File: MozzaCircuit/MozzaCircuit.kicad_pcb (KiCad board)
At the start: 2 copper layers, 183 x 128.1 mm, 174 parts, among them J1 8P8C_both_sides, SW13 SW_ChocV2_rev, SW14 SW_ChocV2_rev, SW15 SW_ChocV2_rev, SW21 SW_ChocV2_rev, SW22 SW_ChocV2_rev, SW23 SW_ChocV2_rev, SW24 SW_ChocV2_rev, SW25 SW_ChocV2_rev, SW31 SW_ChocV2_rev, SW32 SW_ChocV2_rev, SW33 SW_ChocV2_rev, SW34 SW_ChocV2_rev, SW35 SW_ChocV2_rev, SW41 SW_ChocV2_rev, SW42 SW_ChocV2_rev, SW43 SW_ChocV2_rev, SW44 SW_ChocV2_rev, SW51 SW_ChocV2_rev, SW52 SW_ChocV2_rev, SW53 SW_ChocV2_rev, SW54 SW_ChocV2_rev, SW61 SW_ChocV2_rev, SW62 SW_ChocV2_rev, SW63 SW_ChocV2_rev, SW64 SW_ChocV2_rev, SW71 SW_ChocV2_rev, SW72 SW_ChocV2_rev, SW73 SW_ChocV2_rev, SW82 SW_ChocV2_rev, SW83 SW_ChocV2_rev, SW84 SW_ChocV2_rev, U1 MCP23017_ML, U2 MCP23017_ML_NoTP

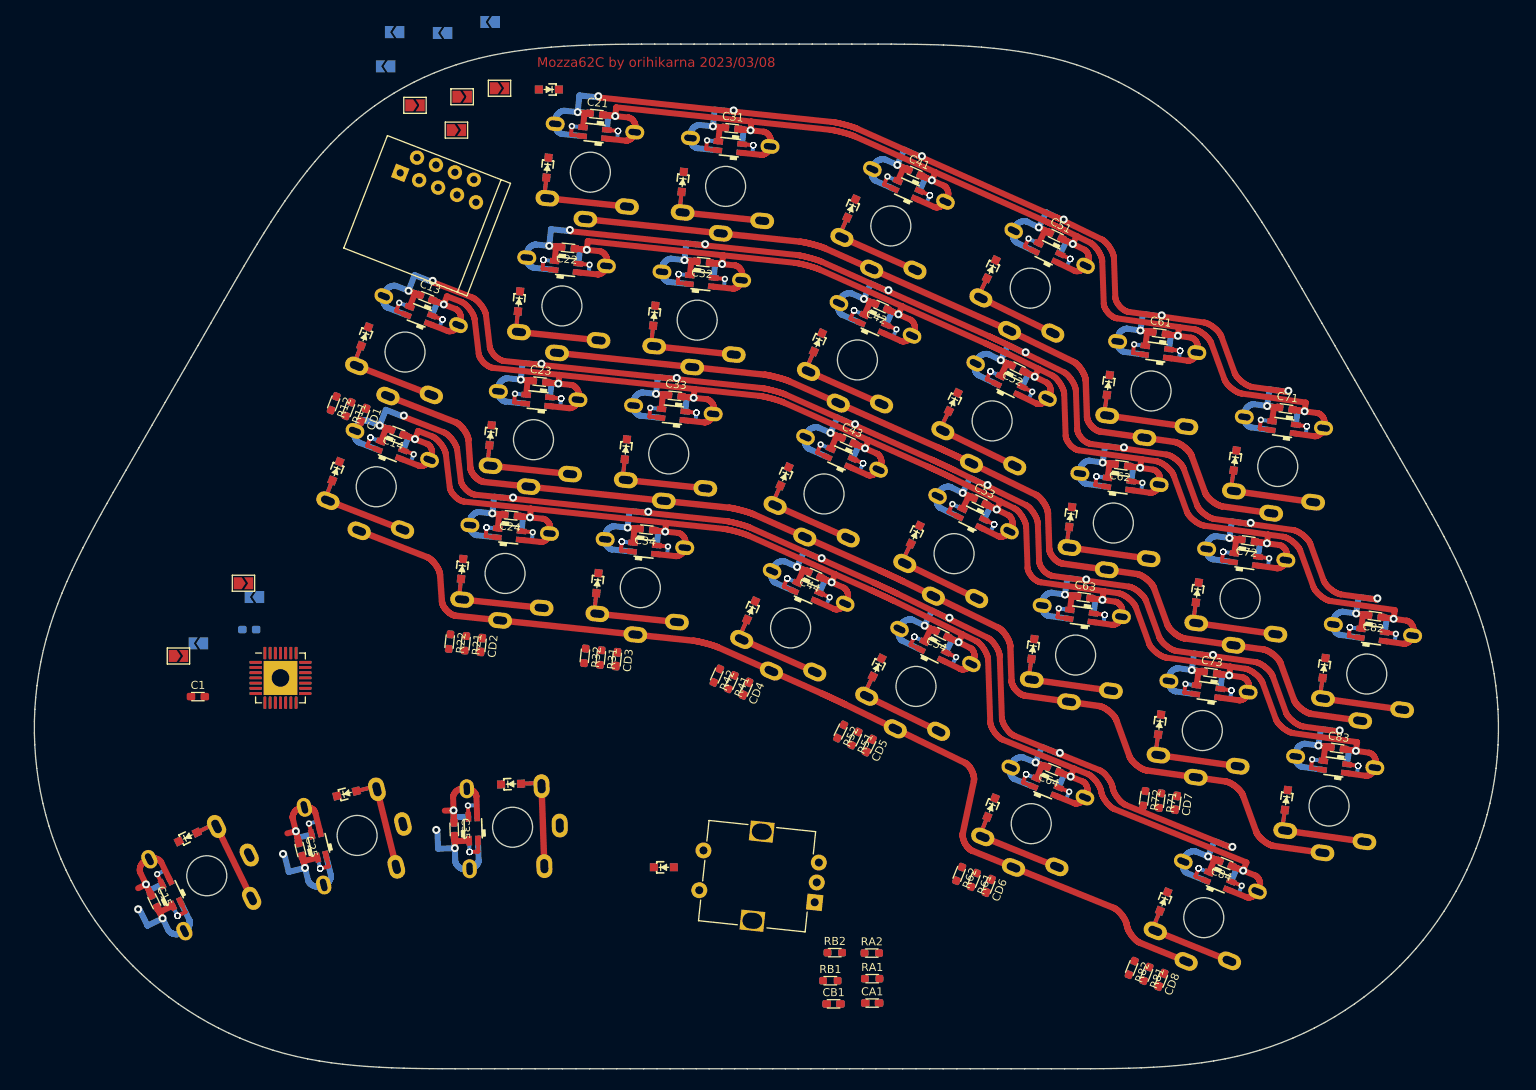
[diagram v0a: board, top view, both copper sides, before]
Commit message: added power cap
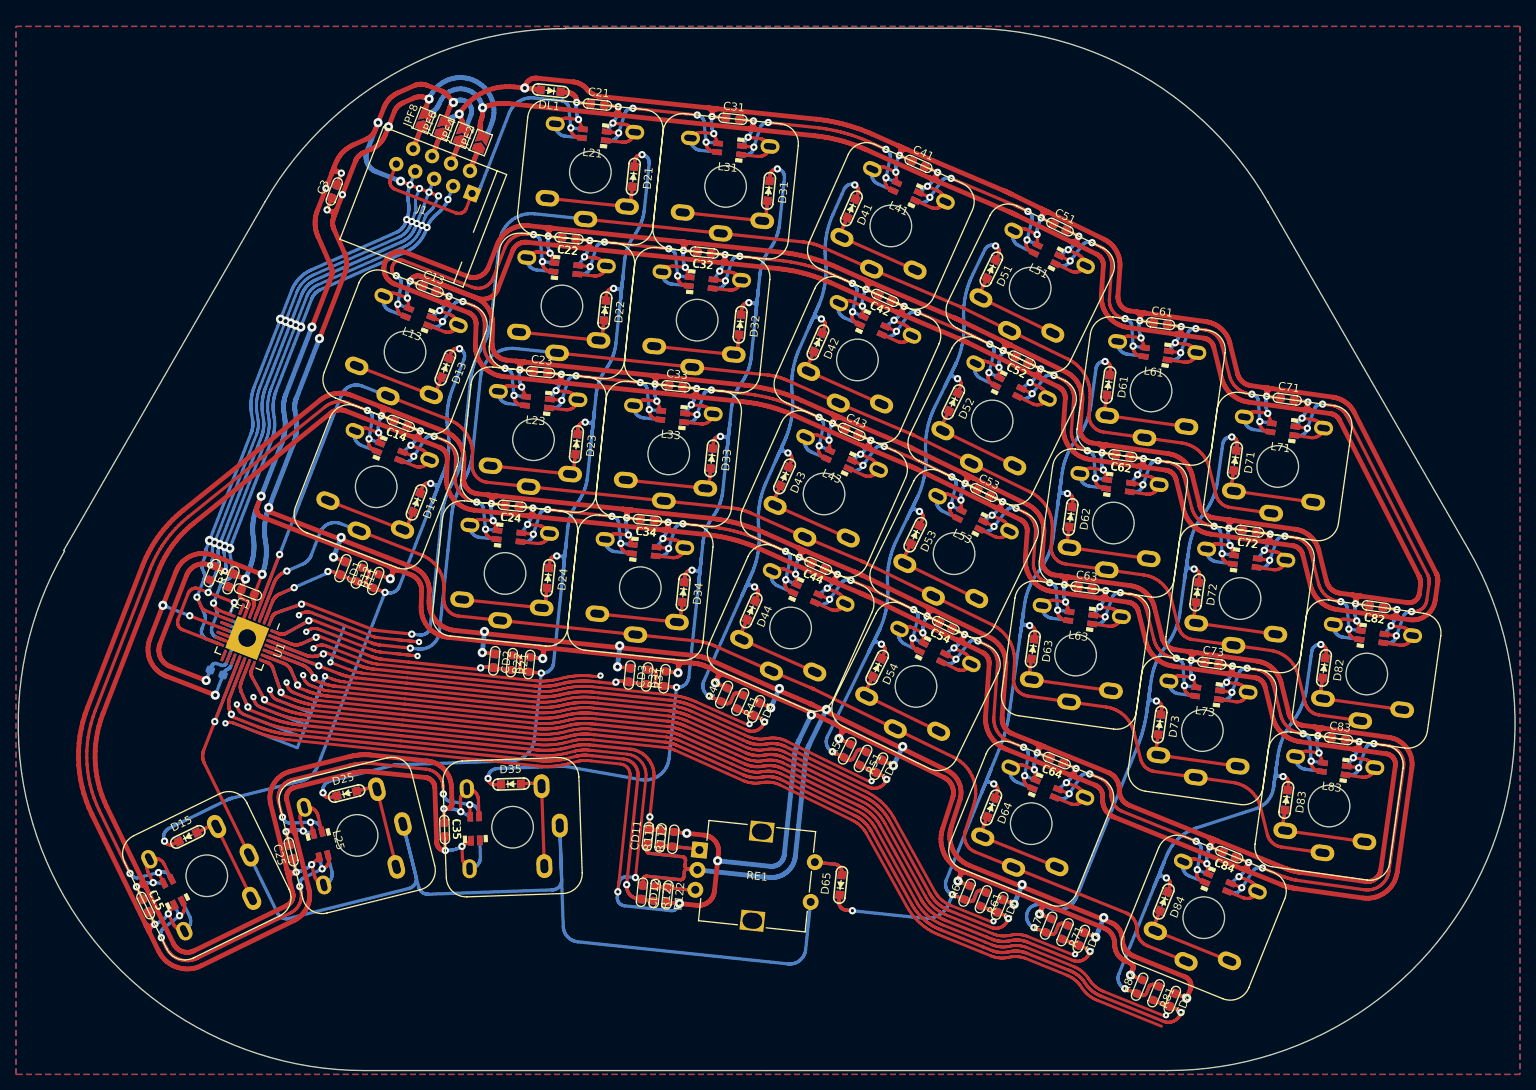
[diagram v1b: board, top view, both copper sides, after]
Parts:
- removed CA1: 33n, 00_KeyParts:C_1608_HandSolder_both_sides
- removed CB1: C_Small, 00_KeyParts:C_1608_HandSolder_both_sides
- removed D45: D_Small, 00_KeyParts:D_SOD-323_both_sides
- removed JPB3, JPB7, JPF3, JPF7: SolderJumper_2_Open, Jumper:SolderJumper-2_P1.3mm_Open_TrianglePad1.0x1.5mm
- removed RA1: 10k, 00_KeyParts:R_1608_HandSolder_both_sides
- removed RA2: 4k7, 00_KeyParts:R_1608_HandSolder_both_sides
- removed RB1, RB2: R_Small_US, 00_KeyParts:R_1608_HandSolder_both_sides
- added C3: C_Small, 00_KeyParts:C_1608_HandSolder_both_sides, F.Cu at (80.3, 40.1)
- added C4: C_Small, 00_KeyParts:C_1608_HandSolder_both_sides, F.Cu at (67.4, 88.7)
- added CD11: 33n, 00_KeyParts:C_1608_HandSolder_both_sides, F.Cu at (119.5, 120.8)
- added CD12: C_Small, 00_KeyParts:C_1608_HandSolder_both_sides, F.Cu at (118.7, 127.7)
- added D65: D_Small, 00_KeyParts:D_SOD-323_both_sides, F.Cu at (143.6, 126.8)
- added R1: 100, 00_KeyParts:R_1608_HandSolder_both_sides, F.Cu at (65.0, 87.8)
- added R111: 10k, 00_KeyParts:R_1608_HandSolder_both_sides, F.Cu at (121.1, 120.9)
- added R112: 4k7, 00_KeyParts:R_1608_HandSolder_both_sides, F.Cu at (122.7, 121.1)
- added R121: R_Small_US, 00_KeyParts:R_1608_HandSolder_both_sides, F.Cu at (120.3, 127.9)
- added R122: R_Small_US, 00_KeyParts:R_1608_HandSolder_both_sides, F.Cu at (121.9, 128.1)
- J1: moved to B.Cu
- JPB2, JPB4, JPB6, JPB8, JPF2, JPF4, JPF6, JPF8: footprint Jumper:SolderJumper-2_P1.3mm_Open_TrianglePad1.0x1.5mm -> 00_KeyParts:SolderJumper-2_P1.3mm_Open_TrianglePad1.0x1.5mm
- moved R12 22.8 mm to (85.5, 88.8), turned to 68.8 degrees
- moved R11 20.7 mm to (83.4, 88.0)
- moved CD7 20.7 mm to (173.7, 133.6), turned to -112 degrees
- moved R71 20.3 mm to (171.6, 132.7), turned to -112 degrees
- moved R72 19.9 mm to (169.6, 131.9), turned to 68 degrees
- moved CD1 19.3 mm to (81.4, 87.2)
- moved JPB6 15.4 mm to (96.3, 33.1), turned to 68.8 degrees
- moved JPB8 15.2 mm to (98.6, 34.0), turned to 68.8 degrees
- moved C1 14.5 mm to (69.5, 90.2), turned to 158.8 degrees
- moved JPB4 14.5 mm to (93.9, 32.2), turned to 68.8 degrees
- moved JPB2 11.2 mm to (91.5, 31.3), turned to 68.8 degrees
- moved D14 10.8 mm to (90.6, 79.0)
- moved D13 10.8 mm to (94.2, 62.2)
- moved D34 10.8 mm to (123.9, 90.2)
- moved D21 10.8 mm to (117.7, 38.3)
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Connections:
- J1 pad 3: Net-(J1-Pad3) -> SCK_SDA
- J1 pad 5: 5VD -> NRST_in
- J1 pad 7: Net-(J1-Pad7) -> SDA_SCK
- JPB2 pad 2: GND -> GNDD
- JPB4 pad 2: GNDD -> 5VD
- JPB6 pad 2: NRST -> GND
- JPB8 pad 2: SDA -> 3V3
- JPF2 pad 2: GND -> GNDD
- JPF4 pad 2: GNDD -> 5VD
- JPF6 pad 2: NRST -> GND
- JPF8 pad 2: SDA -> 3V3
- SW14 pad 4: unconnected-(SW14-Pad4) -> 5VD
- SW14 pad 5: unconnected-(SW14-Pad5) -> GNDD
- SW15 pad 1: Net-(D15-Pad2) -> ROW5
- SW15 pad 2: ROW5 -> Net-(D15-Pad2)
- SW15 pad 3: ROW5 -> Net-(D15-Pad2)
- SW15 pad 4: GNDD -> 5VD
- SW15 pad 5: 5VD -> GNDD
- SW25 pad 4: 5VD -> GNDD
- SW25 pad 5: GNDD -> 5VD
- U1 pad 1: ROW5 -> ROW1
- U1 pad 11: GND -> 3V3
- U1 pad 17: COL1 -> unconnected-(U1-Pad17)
- U1 pad 18: COL2 -> ROW5
- U1 pad 19: COL3 -> COLB
- U1 pad 2: REA -> COL1
- U1 pad 20: COL4 -> COLA
- U1 pad 21: COL5 -> COL8
- U1 pad 22: COL6 -> COL7
- U1 pad 23: COL7 -> COL6
- U1 pad 24: COL8 -> COL5
- U1 pad 25: ROW1 -> COL4
- U1 pad 26: ROW2 -> COL3
- U1 pad 27: ROW3 -> COL2
- U1 pad 28: ROW4 -> ROW2
- U1 pad 3: REB -> ROW4
- U1 pad 4: unconnected-(U1-Pad4) -> ROW3
- U1 pad 8: SCK -> SCK_SDA
- U1 pad 9: SDA -> SDA_SCK
- U2 pad 1: ROW5 -> COL8
- U2 pad 11: 3V3 -> GND
- U2 pad 17: COL1 -> unconnected-(U2-Pad17)
- U2 pad 18: COL2 -> ROW3
- U2 pad 19: COL3 -> ROW4
- U2 pad 2: REA -> COLA
- U2 pad 20: COL4 -> COL1
- U2 pad 21: COL5 -> ROW1
- U2 pad 22: COL6 -> ROW2
- U2 pad 23: COL7 -> COL2
- U2 pad 24: COL8 -> COL3
- U2 pad 25: ROW1 -> COL4
- U2 pad 26: ROW2 -> COL5
- U2 pad 27: ROW3 -> COL6
- U2 pad 28: ROW4 -> COL7
- U2 pad 3: REB -> COLB
- U2 pad 4: unconnected-(U2-Pad4) -> ROW5
- U2 pad 8: SCK -> SDA_SCK
- U2 pad 9: SDA -> SCK_SDA
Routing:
- net GND: track 0.00 -> 1442.4 mm, vias 0 -> 52
- net 3V3: track 0.00 -> 397.3 mm, vias 0 -> 26
- net 5VD: track 1003.8 -> 1331.6 mm, vias 43 -> 62
- net GNDD: track 1051.7 -> 1358.4 mm, vias 48 -> 63
- net Net-(D21-Pad1): track 0.00 -> 161.2 mm, vias 0 -> 6
- net Net-(D31-Pad1): track 0.00 -> 157.7 mm, vias 0 -> 6
- net COL8: track 0.00 -> 145.5 mm, vias 0 -> 2
- net ROW5: track 10.00 -> 153.5 mm, vias 0 -> 1
- net Net-(D61-Pad1): track 0.00 -> 143.2 mm, vias 0 -> 6
- net COL7: track 0.00 -> 130.2 mm, vias 0 -> 2
- net Net-(D51-Pad1): track 0.00 -> 120.3 mm, vias 0 -> 5
- net Net-(D41-Pad1): track 0.00 -> 120.3 mm, vias 0 -> 5
- net COL6: track 0.00 -> 119.4 mm, vias 0 -> 2
- net Net-(D71-Pad1): track 0.00 -> 110.6 mm, vias 0 -> 4
- net Net-(D13-Pad1): track 0.00 -> 110.3 mm, vias 0 -> 4
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- added copper zone on B.Cu, net GND
- added copper zone on F.Cu, net GND
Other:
- board size 183 x 128.1 mm -> 187.1 x 130.3 mm
- board text removed: "Mozza62C by orihikarna 2023/03/08"
